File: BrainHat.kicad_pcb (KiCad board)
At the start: 2 copper layers, 50.6 x 40.3 mm, 50 parts, among them J1 Output, J2 Status, J3 Power, J4 Electrodes, U1 AD8232, U2 ADS1115IDGS, U3 SN74LV1T34DBV

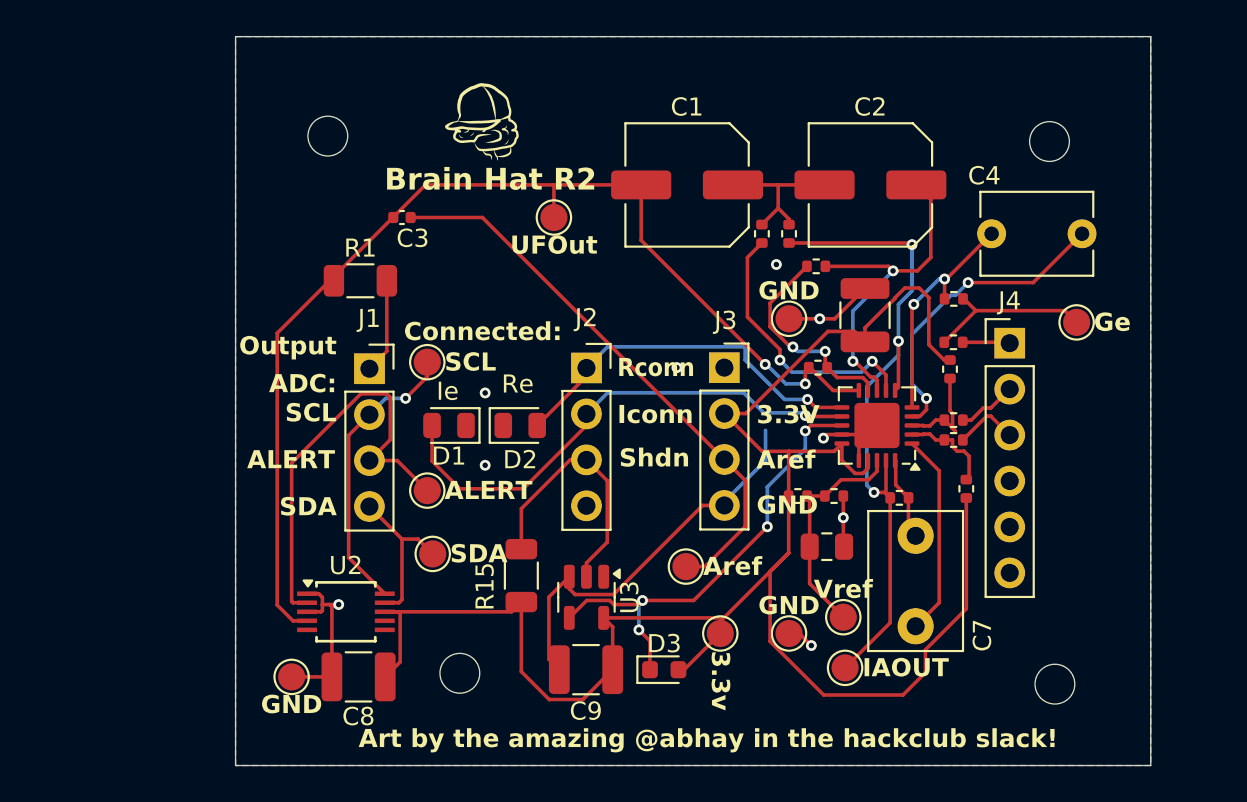
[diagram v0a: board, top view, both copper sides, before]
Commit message: made many a change
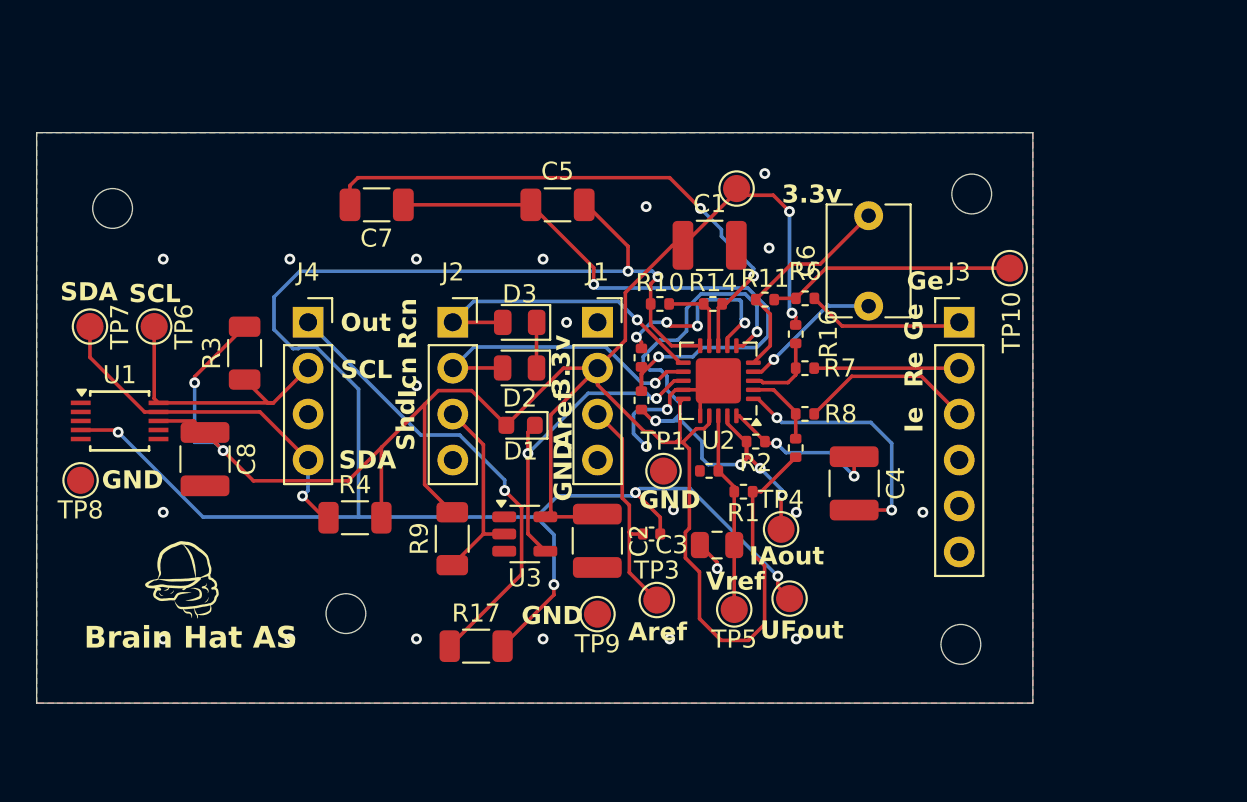
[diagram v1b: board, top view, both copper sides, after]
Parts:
- removed TP12: TestPoint, TestPoint:TestPoint_Pad_D1.5mm
- added R16: 10M±1%, Resistor_SMD:R_0402_1005Metric, F.Cu at (182.0, 81.2)
- added R17: 10k, Resistor_SMD:R_1206_3216Metric, F.Cu at (164.3, 98.4)
- C1, C2: value 220uF -> 100nF; footprint Capacitor_SMD:C_Elec_6.3x5.4 -> Capacitor_SMD:C_1210_3225Metric
- C3: value 14pF -> 10nF; footprint Capacitor_SMD:C_0402_1005Metric -> Capacitor_SMD:C_0805_2012Metric
- C4: value 1nF -> 100nF; footprint Capacitor_THT:C_Disc_D6.0mm_W4.4mm_P5.00mm -> Capacitor_SMD:C_1210_3225Metric
- C5: value 100nF -> 220uF; footprint Capacitor_SMD:C_1210_3225Metric -> Capacitor_SMD:C_1206_3216Metric
- C6: value 10nF -> 1nF; footprint Capacitor_SMD:C_0805_2012Metric -> Capacitor_THT:C_Disc_D6.0mm_W4.4mm_P5.00mm
- C7: value 100nF -> 220uF; footprint Capacitor_THT:C_Disc_D7.5mm_W5.0mm_P5.00mm -> Capacitor_SMD:C_1206_3216Metric
- C9: value 100nF -> 14pF; footprint Capacitor_SMD:C_1210_3225Metric -> Capacitor_SMD:C_0402_1005Metric
- D1: value XL-2012UWC -> XL-1608UBC-04; footprint LED_SMD:LED_0805_2012Metric -> LED_SMD:LED_0603_1608Metric
- D3: value XL-1608UBC-04 -> XL-2012UWC; footprint LED_SMD:LED_0603_1608Metric -> LED_SMD:LED_0805_2012Metric
- J1: value Output -> Power
- J3: value Power -> Electrodes; footprint Connector_PinSocket_2.54mm:PinSocket_1x04_P2.54mm_Vertical -> Connector_PinHeader_2.54mm:PinHeader_1x06_P2.54mm_Vertical
- J4: value Electrodes -> Output; footprint Connector_PinHeader_2.54mm:PinHeader_1x06_P2.54mm_Vertical -> Connector_PinSocket_2.54mm:PinSocket_1x04_P2.54mm_Vertical
- R1, R15: value 10k -> 10M±1%; footprint Resistor_SMD:R_1206_3216Metric -> Resistor_SMD:R_0402_1005Metric
- R10: value 10M±1% -> 604
- R11: value 10M±1% -> 412k
- R12: value 1.58M -> 1.2M
- R13: value 330k -> 1.2M
- R14: value 330k -> 1k
- R2: value 1.2M -> 1.58M
- R3: value 1.2M -> 10k; footprint Resistor_SMD:R_0402_1005Metric -> Resistor_SMD:R_1206_3216Metric
- R4: value 1k -> 10k; footprint Resistor_SMD:R_0402_1005Metric -> Resistor_SMD:R_1206_3216Metric
- R5: value 412k -> 10M±1%
- R6: value 604 -> 330k
- R8: value 10M±1% -> 330k
- R9: value 10M±1% -> 10k; footprint Resistor_SMD:R_0402_1005Metric -> Resistor_SMD:R_1206_3216Metric
- U1: value AD8232 -> ADS1113IDGS; footprint Package_CSP:LFCSP-20-1EP_4x4mm_P0.5mm_EP2.5x2.5mm -> Package_SO:TSSOP-10_3x3mm_P0.5mm
- U2: value ADS1115IDGS -> AD8232; footprint Package_SO:TSSOP-10_3x3mm_P0.5mm -> Package_CSP:LFCSP-20-1EP_4x4mm_P0.5mm_EP2.5x2.5mm
- moved U1 41.9 mm to (144.6, 86.0), turned to 0 degrees
- moved H4 39.4 mm to (157.1, 96.6)
- moved J4 38.8 mm to (155.0, 80.5)
- moved TP7 38.8 mm to (142.9, 80.7), turned to -90 degrees
- moved C7 37.8 mm to (158.8, 74.0), turned to 180 degrees
- moved H1 35.7 mm to (191.7, 73.4)
- moved TP8 33.8 mm to (142.4, 89.2), turned to 180 degrees
- moved H3 32.1 mm to (144.2, 74.2)
- moved R3 30.8 mm to (151.5, 82.2)
- moved R4 29.0 mm to (157.6, 91.3)
- moved H2 28.2 mm to (191.1, 98.3)
- moved TP11 27.9 mm to (181.6, 95.8)
- moved C3 25.1 mm to (177.6, 92.8)
- moved C2 24.8 mm to (171.0, 92.6), turned to -90 degrees
- moved U2 24.2 mm to (177.7, 83.7), turned to 180 degrees
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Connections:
- C1 pad 1: Net-(C5-Pad1) -> +3.3V
- C1 pad 2: UFOUT1 -> GND
- C2 pad 1: REFOUT1 -> +3.3V
- C2 pad 2: Net-(C5-Pad1) -> GND
- C3 pad 1: Aref -> Vref
- C3 pad 2: UFOUT1 -> GND
- C4 pad 1: RLDFB1 -> HPSENSE1
- C4 pad 2: RLD1 -> HPDRIVE1
- C5 pad 1: +3.3V -> Net-(C5-Pad1)
- C5 pad 2: GND -> UFOUT1
- C6 pad 1: Vref -> RLDFB1
- C6 pad 2: GND -> RLD1
- C7 pad 1: HPDRIVE1 -> Net-(C5-Pad1)
- C7 pad 2: HPSENSE1 -> REFOUT1
- C9 pad 1: +3.3V -> Aref
- C9 pad 2: GND -> UFOUT1
- D1 pad 1: GND -> shutdown
- D1 pad 2: connectedI -> +3.3V
- D2 pad 2: connectedR -> connectedI
- D3 pad 1: shutdown -> GND
- D3 pad 2: +3.3V -> connectedR
- J1 pad 1: 1o -> unconnected-(J1-Pin_1-Pad1)
- J1 pad 2: SCL -> +3.3V
- J1 pad 3: ALERT -> Aref
- J1 pad 4: SDA -> GND
- J3 pad 1: unconnected-(J1-Pin_1-Pad1) -> Net-(J3-Pin_1)
- J3 pad 2: +3.3V -> /E-
- J3 pad 3: Aref -> /E+
- J3 pad 4: GND -> unconnected-(J3-Pin_4-Pad4)
- J4 pad 1: Net-(J3-Pin_1) -> 1o
- J4 pad 2: /E- -> SCL
- J4 pad 3: /E+ -> ALERT
- J4 pad 4: unconnected-(J3-Pin_4-Pad4) -> SDA
- R1 pad 1: 1o -> +3.3V
- R1 pad 2: UFOUT1 -> Vref
- R10 pad 1: +3.3V -> UFOUT1
- R10 pad 2: Vref -> OPAMP-1
- R11 pad 1: +3.3V -> RLD1
- R11 pad 2: IN+ -> Ge
- R12 pad 1: HPSENSE1 -> IAOUT1
- R12 pad 2: IAOUT1 -> Net-(C5-Pad1)
- R13 pad 1: IN- -> Net-(C5-Pad1)
- R13 pad 2: /E- -> OPAMP+1
- R14 pad 1: IN+ -> OPAMP-1
- R14 pad 2: /E+ -> REFOUT1
- R15 pad 1: 5Vshutdown -> +3.3V
- R15 pad 2: +3.3V -> IN+
- R2 pad 1: Net-(C5-Pad1) -> HPSENSE1
- R2 pad 2: OPAMP+1 -> IAOUT1
- R3 pad 1: IAOUT1 -> SCL
- R3 pad 2: Net-(C5-Pad1) -> +3.3V
- R4 pad 1: OPAMP-1 -> SDA
- R4 pad 2: REFOUT1 -> +3.3V
- R5 pad 1: RLD1 -> Vref
- R5 pad 2: Ge -> GND
- R6 pad 1: UFOUT1 -> Ge
- R6 pad 2: OPAMP-1 -> Net-(J3-Pin_1)
- R7 pad 1: Ge -> IN-
- R7 pad 2: Net-(J3-Pin_1) -> /E-
- R8 pad 1: +3.3V -> IN+
- R8 pad 2: IN- -> /E+
- R9 pad 1: Vref -> 5Vshutdown
- R9 pad 2: GND -> +3.3V
- TP1 pad 1: UFOUT1 -> GND
- TP10 pad 1: GND -> Ge
- TP11 pad 1: GND -> UFOUT1
- TP2 pad 1: SCL -> +3.3V
- TP3 pad 1: GND -> Aref
- TP4 pad 1: Ge -> IAOUT1
- TP5 pad 1: ALERT -> Vref
- TP6 pad 1: SDA -> SCL
- TP7 pad 1: +3.3V -> SDA
- TP8 pad 1: Aref -> GND
- TP9 pad 1: Vref -> GND
- U1 pad 1: HPDRIVE1 -> GND
- U1 pad 10: UFOUT1 -> SCL
- U1 pad 2: IN+ -> unconnected-(U1-Pad2)
- U1 pad 3: IN- -> GND
- U1 pad 4: RLDFB1 -> UFOUT1
- U1 pad 5: RLD1 -> GND
- U1 pad 6: IAOUT1 -> unconnected-(U1-Pad6)
- U1 pad 7: OPAMP+1 -> unconnected-(U1-Pad7)
- U1 pad 8: REFOUT1 -> +3.3V
- U1 pad 9: OPAMP-1 -> SDA
- U2 pad 1: GND -> HPDRIVE1
- U2 pad 10: SCL -> UFOUT1
- U2 pad 2: ALERT -> IN+
- U2 pad 3: GND -> IN-
- U2 pad 4: UFOUT1 -> RLDFB1
- U2 pad 5: unconnected-(U1-AIN1-Pad5) -> RLD1
- U2 pad 6: unconnected-(U1-AIN2-Pad6) -> IAOUT1
- U2 pad 7: unconnected-(U1-AIN3-Pad7) -> OPAMP+1
- U2 pad 8: +3.3V -> REFOUT1
- U2 pad 9: SDA -> OPAMP-1
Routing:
- net UFOUT1: track 62.0 -> 104.0 mm, vias 2 -> 6
- net GND: track 43.3 -> 12.3 mm, vias 9 -> 22
- net Net-(C5-Pad1): track 8.77 -> 34.8 mm, vias 0 -> 2
- net ALERT: track 23.5 -> 0.00 mm
- net 1o: track 5.26 -> 25.7 mm, vias 0 -> 1
- net Aref: track 31.3 -> 12.4 mm
- net +3.3V: track 103.7 -> 122.1 mm, vias 0 -> 4
- net REFOUT1: track 18.8 -> 31.1 mm
- net SDA: track 8.95 -> 19.9 mm, vias 0 -> 1
- net connectedI: track 27.7 -> 17.1 mm
- net RLDFB1: track 17.2 -> 7.92 mm, vias 2 -> 1
- net shutdown: track 25.7 -> 18.0 mm, vias 4 -> 2
- net OPAMP-1: track 11.6 -> 4.35 mm, vias 2 -> 0
- net /E+: track 3.57 -> 9.75 mm
- net Net-(J3-Pin_1): track 2.55 -> 8.43 mm
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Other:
- board size 50.6 x 40.3 mm -> 55.1 x 31.5 mm
- board text added: "Brain Hat AS"
- board text added: "IAout"
- board text added: "Icn"
- board text added: "Out"
- board text added: "Rcn"
- board text added: "Shd"
- board text added: "UFout"
- board text removed: "3.3V"
- board text removed: "ADC: SCL"
- board text removed: "ALERT"
- board text removed: "Art by the amazing @abhay in the hackclub slack!"
- board text removed: "Brain Hat R2"
- board text removed: "Connected:"
- board text removed: "IAOUT"
- board text removed: "Iconn"
- board text removed: "Output"
- board text removed: "Rconn"
- board text removed: "Shdn"
- board text removed: "UFOut"
